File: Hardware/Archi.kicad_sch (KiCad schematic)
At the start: 19 parts, among them J4 Power, J5 Analog, J6 Digital/PWM, J7 Digital/PWM, U5 SWITCH

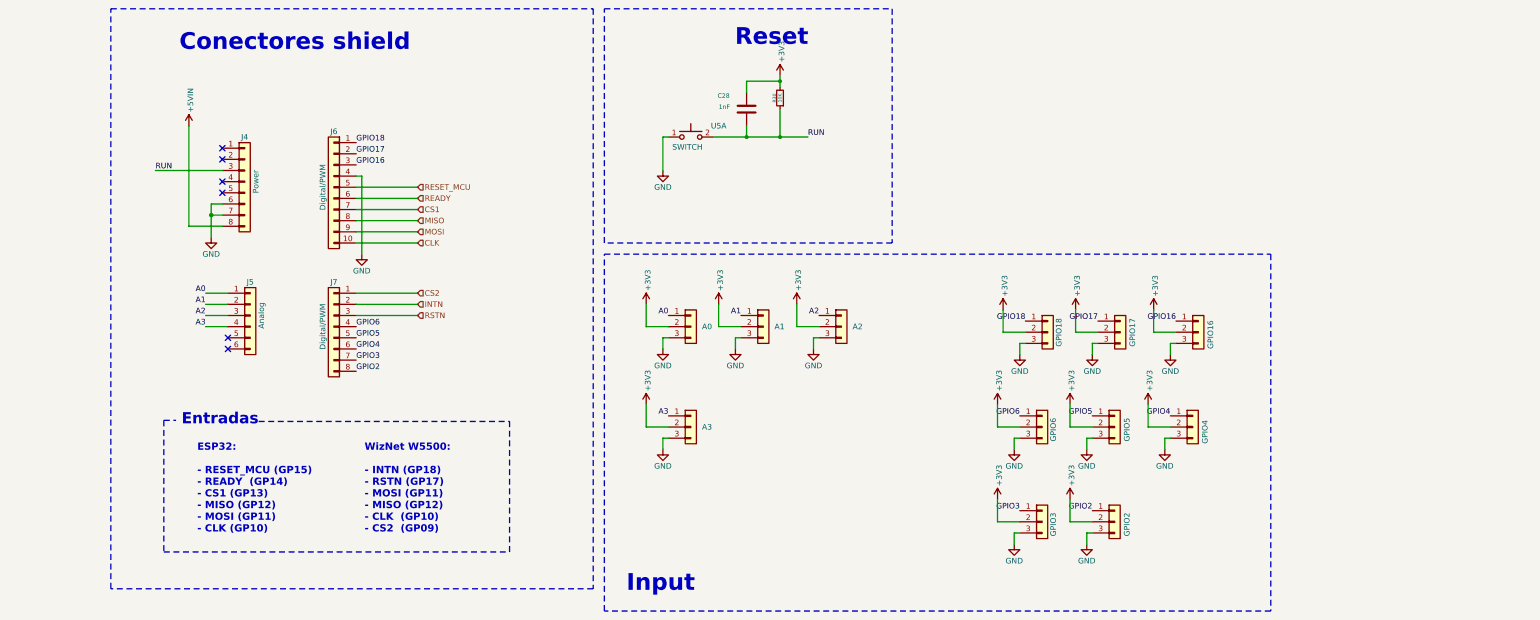
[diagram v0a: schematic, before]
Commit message: .add digikey
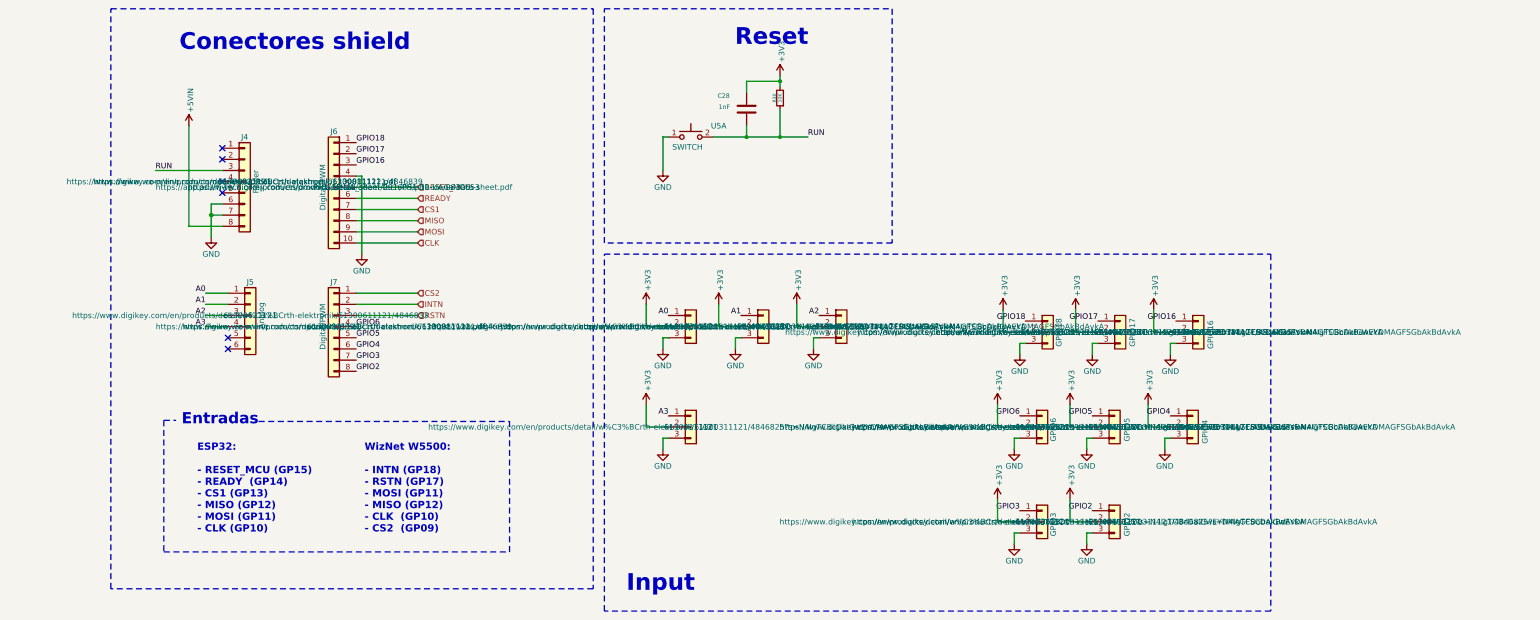
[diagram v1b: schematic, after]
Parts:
- A0, A1, A2, A3, GPIO16, GPIO17, GPIO18, GPIO2, GPIO3, GPIO4, GPIO5, GPIO6: PartNumber (none) -> 61300311121; PurchaseLink (none) -> https://www.digikey.com/en/products/detail/w%C3%BCrth-elekt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
- J4, J7: PartNumber (none) -> 61300811121; PurchaseLink (none) -> https://www.digikey.com/en/products/detail/w%C3%BCrth-elekt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
- J5: PartNumber (none) -> 61300611121; PurchaseLink (none) -> https://www.digikey.com/en/products/detail/w%C3%BCrth-elekt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
- J6: PartNumber (none) -> PH1-10-UA; PurchaseLink (none) -> https://www.digikey.com/en/products/detail/adam-tech/PH1-10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
